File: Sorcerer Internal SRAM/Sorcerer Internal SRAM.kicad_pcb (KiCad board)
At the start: 2 copper layers, 66.1 x 49.6 mm, 21 parts, among them J1 Sorcerer interface, J2 HIGH RAM, J3 LOW RAM, U1 74LS138, U2 CY7C185, U3 CY62256, U4 CY62256

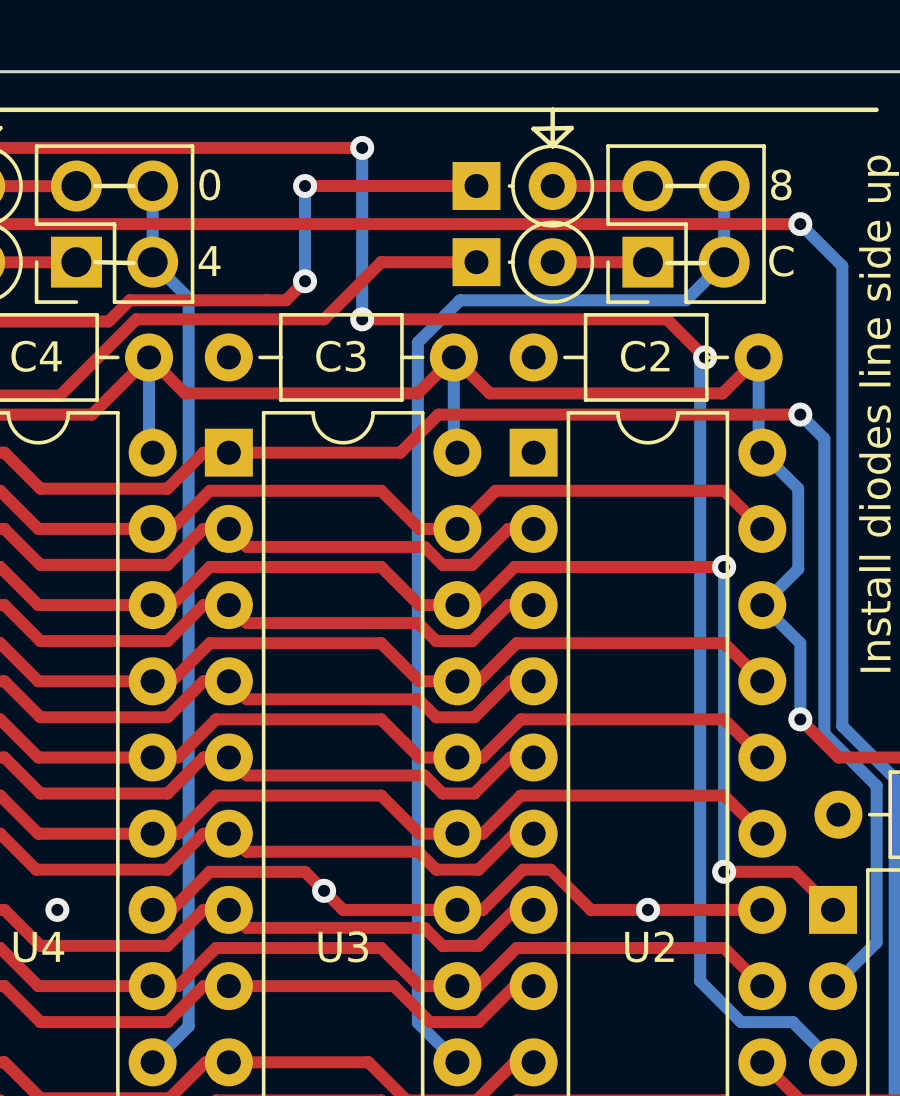
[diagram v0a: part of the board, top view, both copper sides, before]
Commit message: added gerbers for boards I had made
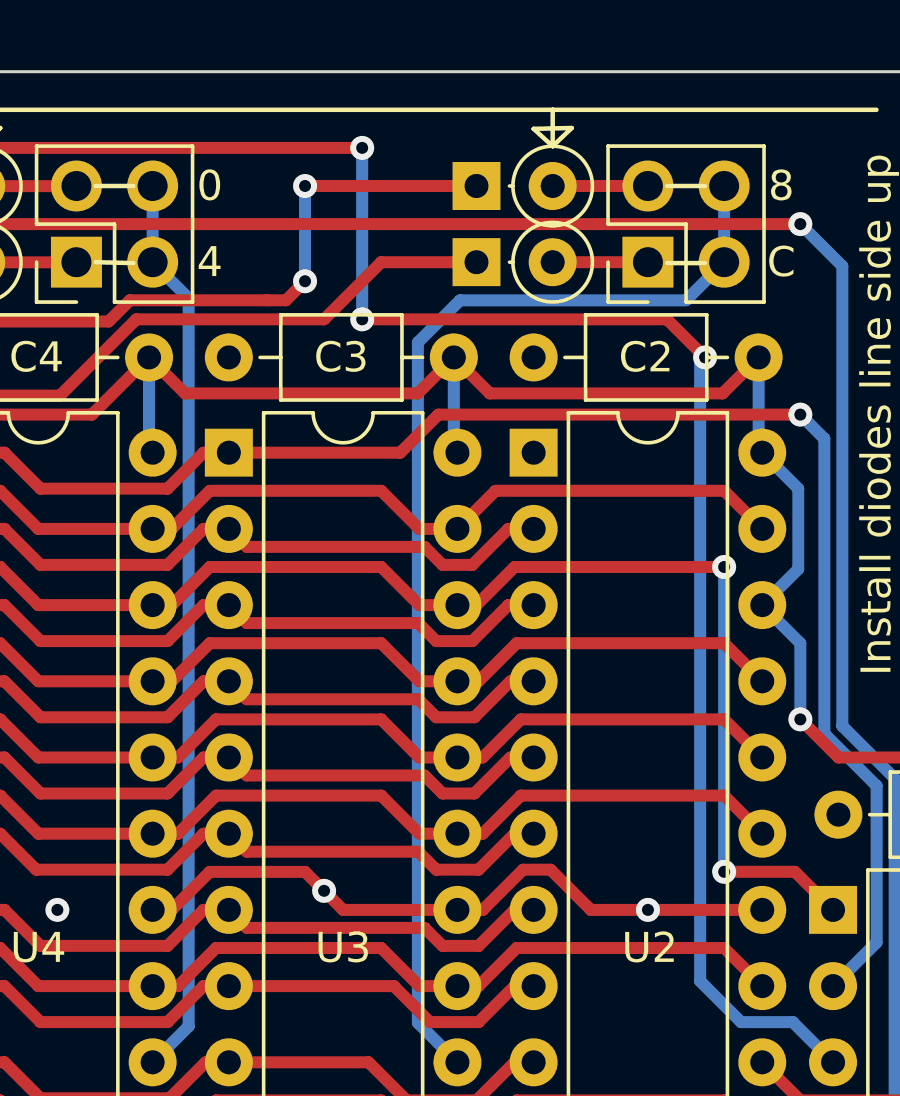
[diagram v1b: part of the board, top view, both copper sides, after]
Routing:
- net RAM 8000-BFFF: track 30.7 -> 29.3 mm
- net GND: track 26.2 -> 25.0 mm
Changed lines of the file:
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@@
       (layerselection 0x00010fc_ffffffff)
       (disableapertmacros false)
-      (usegerberextensions false)
-      (usegerberattributes true)
-      (usegerberadvancedattributes true)
-      (creategerberjobfile true)
+      (usegerberextensions true)
+      (usegerberattributes false)
+      (usegerberadvancedattributes false)
+      (creategerberjobfile false)
       (svguseinch false)
       (svgprecision 6)
@@
       (plotinvisibletext false)
       (sketchpadsonfab false)
-      (subtractmaskfromsilk false)
+      (subtractmaskfromsilk true)
       (outputformat 1)
       (mirror false)
-      (drillshape 1)
+      (drillshape 0)
       (scaleselection 1)
-      (outputdirectory "")
+      (outputdirectory "Sorcerer Internal SRAM gerbers/")
     )
   )
@@
   (segment (start 121.285 69.85) (end 118.745 69.85) (width 0.4) (layer "F.Cu") (net 2))
   (segment (start 142.875 82.55) (end 139.065 82.55) (width 0.4) (layer "F.Cu") (net 2))
-  (segment (start 142.875 82.55) (end 141.74363 82.55) (width 0.4) (layer "F.Cu") (net 2))
   (segment (start 134.617892 81.282108) (end 133.35 82.55) (width 0.4) (layer "F.Cu") (net 2))
   (segment (start 138.43 81.915) (end 137.797108 81.282108) (width 0.4) (layer "F.Cu") (net 2))
@@
   (segment (start 143.51 58.42) (end 137.795 58.42) (width 0.4) (layer "F.Cu") (net 5))
   (segment (start 124.598145 62.935489) (end 131.250295 62.935489) (width 0.4) (layer "F.Cu") (net 5))
-  (segment (start 142.02715 58.42) (end 143.51 58.42) (width 0.4) (layer "F.Cu") (net 5))
   (segment (start 122.763634 64.77) (end 124.598145 62.935489) (width 0.4) (layer "F.Cu") (net 5))
   (segment (start 118.745 64.77) (end 122.763634 64.77) (width 0.4) (layer "F.Cu") (net 5))
